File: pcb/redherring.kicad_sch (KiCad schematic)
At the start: 214 parts, among them J2 OLED, SW3 Rotary_Encoder_Switch, U1 ATmega32A-PU, Y1 16Mhz

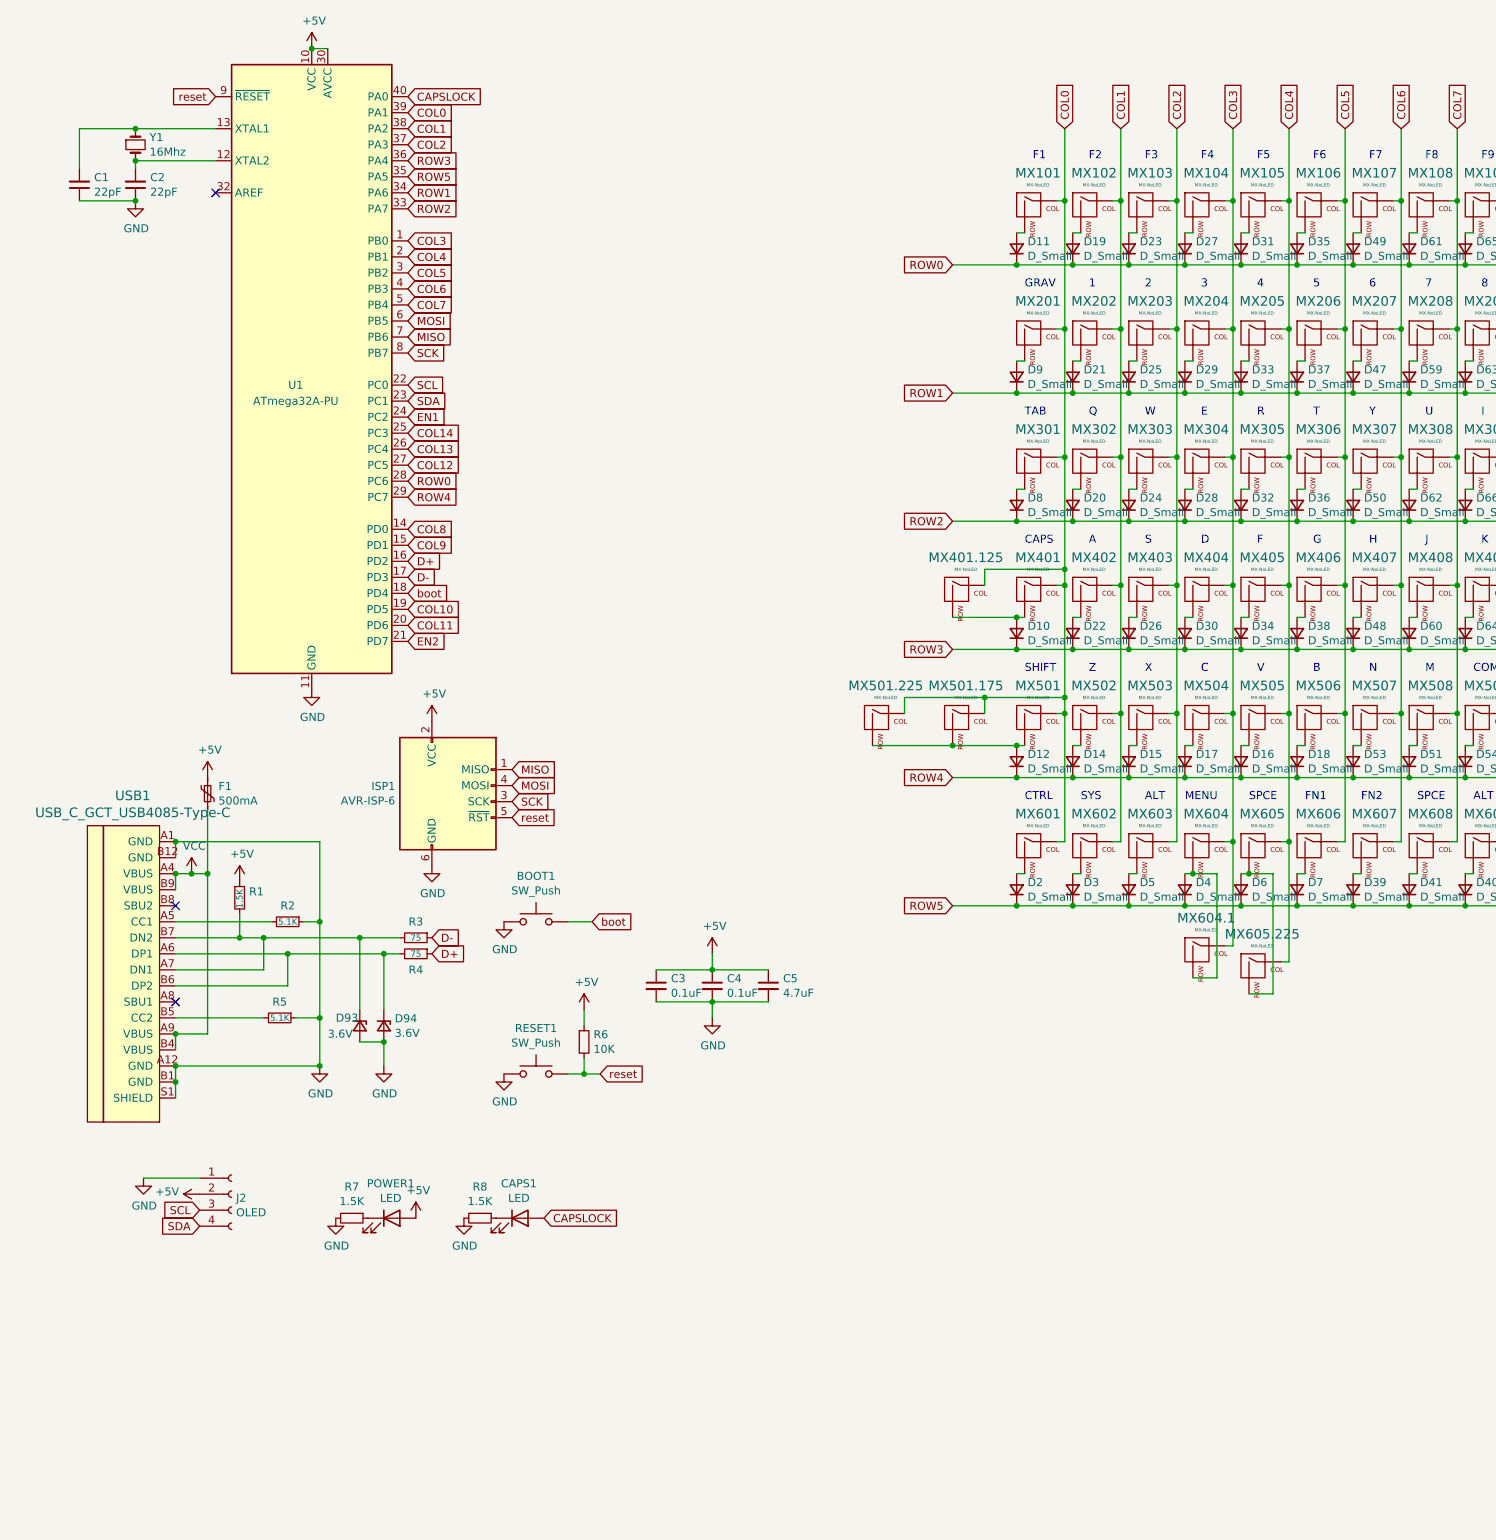
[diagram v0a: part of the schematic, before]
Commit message: Initianl checkin of blueherring.
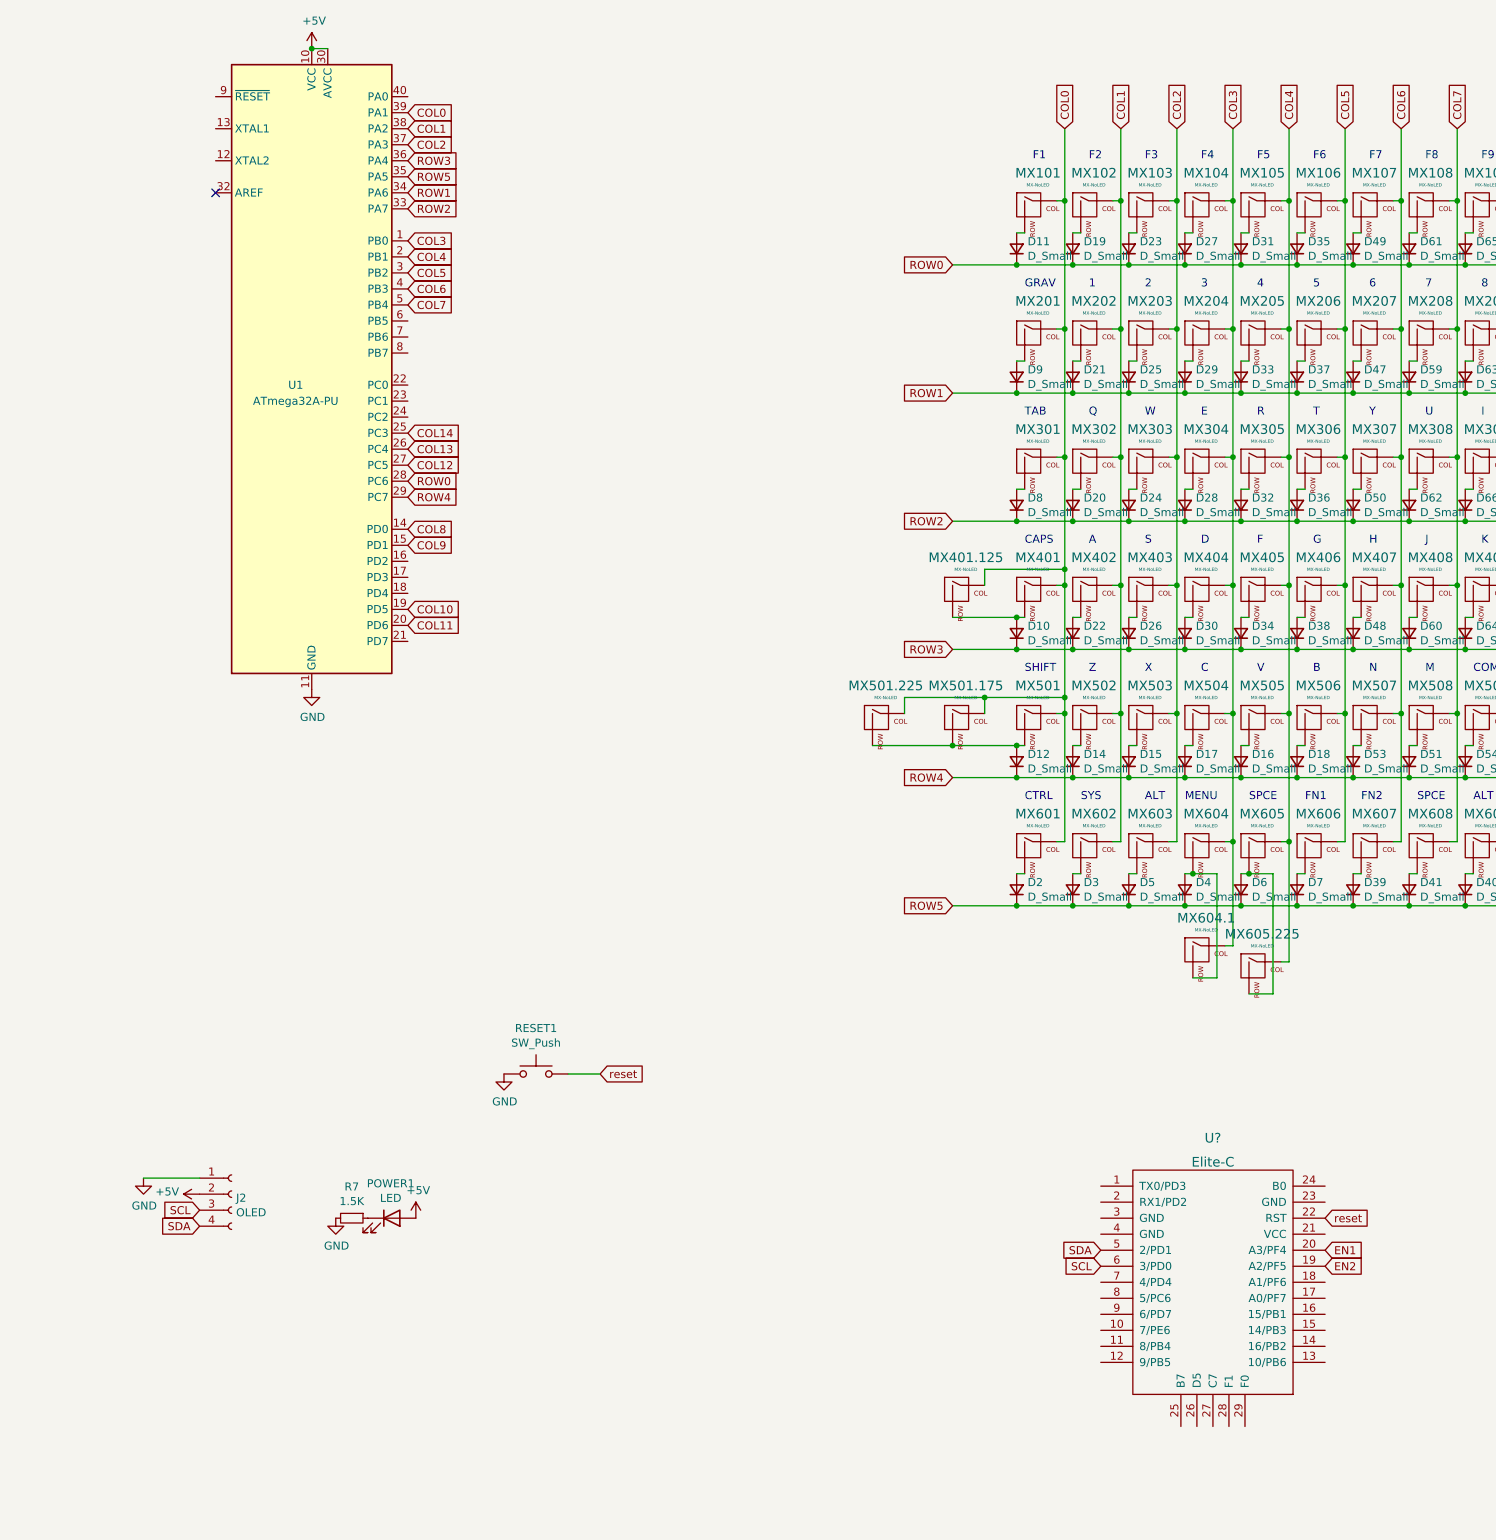
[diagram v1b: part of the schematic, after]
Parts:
- removed BOOT1: SW_Push, Button_Switch_THT:SW_PUSH_6mm, symbol Switch:SW_Push
- removed C1, C2: 22pF, Capacitor_THT:C_Disc_D3.0mm_W2.0mm_P2.50mm, symbol Device:C_Small
- removed C3, C4: 0.1uF, Capacitor_THT:C_Disc_D4.3mm_W1.9mm_P5.00mm, symbol Device:C_Small
- removed C5: 4.7uF, Capacitor_THT:CP_Radial_D4.0mm_P1.50mm, symbol Device:C_Small
- removed CAPS1: LED, LED_THT:LED_D3.0mm_Clear, symbol Device:LED
- removed D93, D94: 3.6V, Diode_THT:D_DO-35_SOD27_P7.62mm_Horizontal, symbol Device:D_Zener_Small
- removed F1: 500mA, cftkb:polyfuse_5.1mm, symbol Device:Polyfuse_Small
- removed ISP1: AVR-ISP-6, Connector_PinHeader_2.54mm:PinHeader_2x03_P2.54mm_Vertical, symbol Connector:AVR-ISP-6
- removed R1, R8: 1.5K, Resistor_THT:R_Axial_DIN0204_L3.6mm_D1.6mm_P5.08mm_Horizontal, symbol Device:R_Small
- removed R2, R5: 5.1K, Resistor_THT:R_Axial_DIN0204_L3.6mm_D1.6mm_P5.08mm_Horizontal, symbol Device:R_Small
- removed R3, R4: 75, Resistor_THT:R_Axial_DIN0204_L3.6mm_D1.6mm_P5.08mm_Horizontal, symbol Device:R_Small
- removed R6: 10K, Resistor_THT:R_Axial_DIN0204_L3.6mm_D1.6mm_P5.08mm_Horizontal, symbol Device:R_Small
- removed USB1: USB_C_GCT_USB4085-Type-C, Type-C:USB_C_GCT_USB4085, symbol redherring-rescue:USB_C_GCT_USB4085-Type-C
- removed Y1: 16Mhz, Crystal:Crystal_HC49-4H_Vertical, symbol Device:Crystal_Small
- added U?: Elite-C, symbol keebio:Elite-C
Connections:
- net EN1: now also U?.20 (A3/PF4); no longer U1.24 (PC2)
- net EN2: now also U?.19 (A2/PF5); no longer U1.21 (PD7)
- net SCL: now also U?.6 (3/PD0); no longer U1.22 (PC0)
- net SDA: now also U?.5 (2/PD1); no longer U1.23 (PC1)
- net reset: now also U?.22 (RST); no longer U1.9 (~{RESET})
- net CAPSLOCK: no longer names the net of U1.40 (PA0)
- net D+: no longer names the net of U1.16 (PD2)
- net D-: no longer names the net of U1.17 (PD3)
- net MISO: no longer names the net of U1.7 (PB6)
- net MOSI: no longer names the net of U1.6 (PB5)
- net SCK: no longer names the net of U1.8 (PB7)
- net boot: no longer names the net of U1.18 (PD4)
- no-connect marks 3 -> 1
